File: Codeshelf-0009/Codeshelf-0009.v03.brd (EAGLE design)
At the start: 28 parts, among them J1 CONTACT-SPRING-S7071-42R, J2 CONTACT-SPRING-S7071-42R, J3 CONTACT-SPRING-S7071-42R, J4 CONTACT-SPRING-S7071-42R, U1 MC9S08QG-DT, U2 LED5060A, U3 RS485SOIC, U4 CAT9552

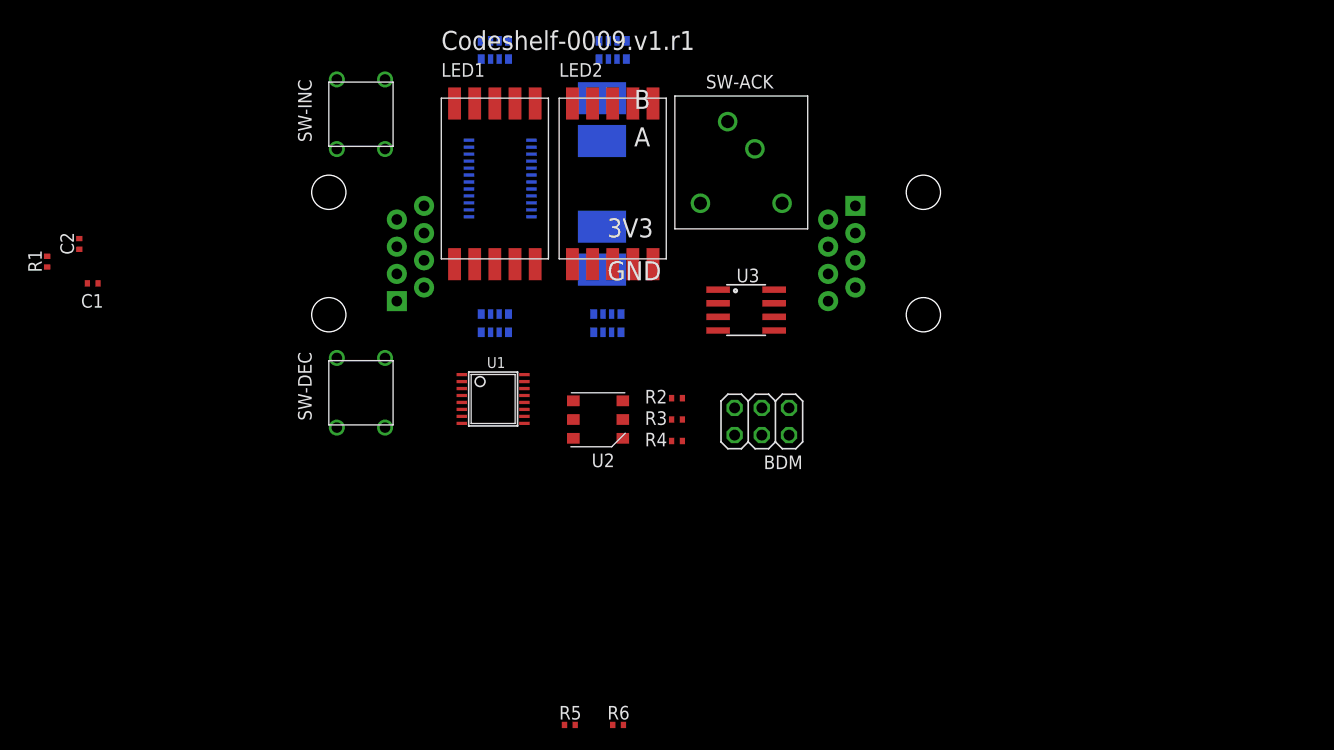
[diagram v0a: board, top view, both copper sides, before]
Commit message: Started new SlotFlex Layout
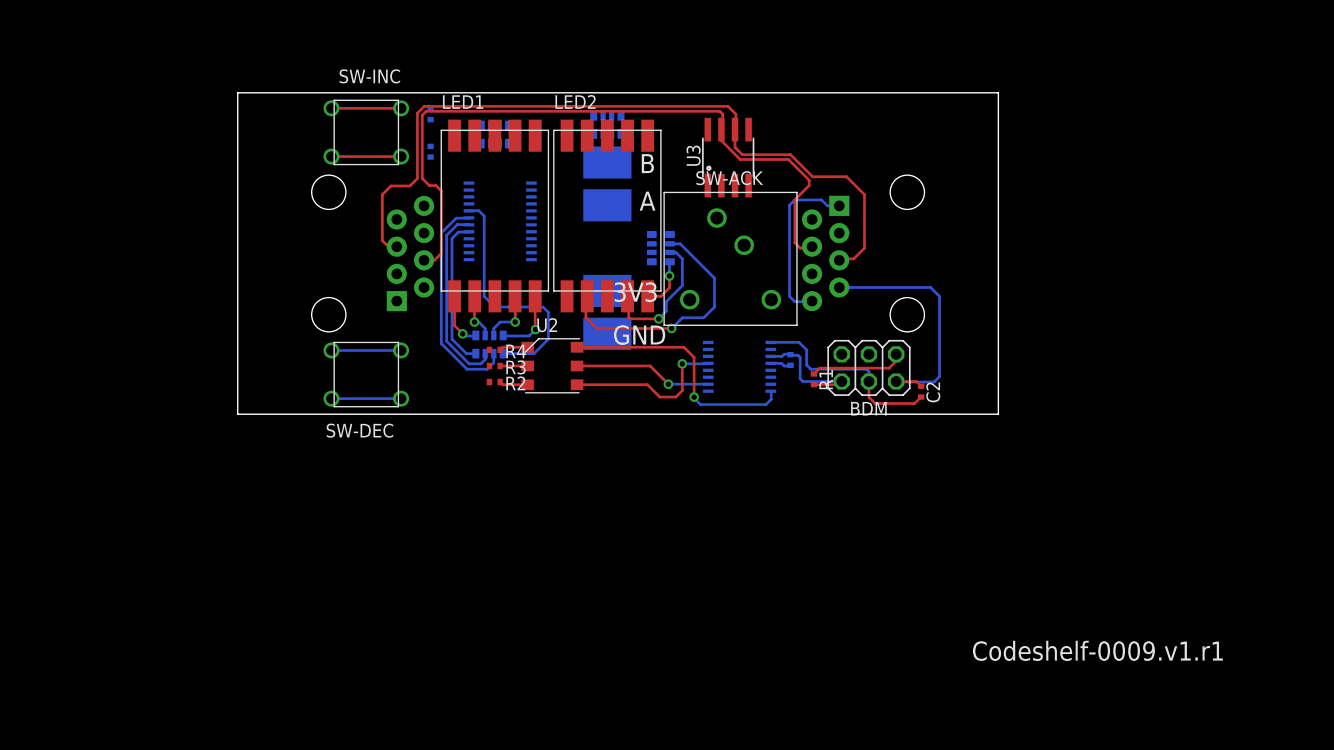
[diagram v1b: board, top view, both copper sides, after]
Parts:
- moved C2 79.8 mm to (44.8, -0.89), turned to 270 degrees
- moved R1 72.4 mm to (34.8, 0.26), turned to 270 degrees
- moved C1 65.5 mm to (32.6, 2.06), flipped to the bottom, turned to 270 degrees
- moved R5 58.5 mm to (-1.00, 25.0), flipped to the bottom, turned to 90 degrees
- moved R6 56.3 mm to (-1.00, 21.5), flipped to the bottom, turned to 90 degrees
- moved U1 23.2 mm to (27.8, 1.42), flipped to the bottom
- moved R4 19.0 mm to (5.00, 3.00), turned to 180 degrees
- moved R3 17.7 mm to (5.00, 1.50), turned to 180 degrees
- moved R2 17.1 mm to (5.00, 0.00), turned to 180 degrees
- moved U3 14.3 mm to (26.8, 20.9), turned to 0 degrees
- moved BDM 11.2 mm to (37.4, 2.59)
- moved SW-ACK 9.06 mm to (27.0, 11.5)
- moved R.D2D 8.60 mm to (20.5, 12.5), turned to 90 degrees
- moved R.D2B 7.90 mm to (5.00, 23.1)
- moved R.D2A 7.02 mm to (15.5, 24.0)
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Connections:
- net A renamed 485_P
- net B renamed 485_N
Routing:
- net 485_P: track 0.00 -> 71.0 mm
- net 485_N: track 0.00 -> 64.7 mm
- net GND: track 0.00 -> 38.9 mm
- net +3V3: track 0.00 -> 27.6 mm
- net N$7: track 0.00 -> 23.5 mm, vias 0 -> 1
- net N$24: track 0.00 -> 23.5 mm, vias 0 -> 1
- net N$38: track 0.00 -> 23.0 mm
- net N$37: track 0.00 -> 20.5 mm
- net N$23: track 0.00 -> 18.9 mm
- net N$36: track 0.00 -> 17.6 mm
- net N$5: track 0.00 -> 15.5 mm, vias 0 -> 1
- net N$35: track 0.00 -> 14.0 mm
- net N$6: track 0.00 -> 13.0 mm, vias 0 -> 1
- net N$22: track 0.00 -> 12.8 mm, vias 0 -> 1
- net N$9: track 0.00 -> 8.80 mm
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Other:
- board outline added: 71 x 30 mm
